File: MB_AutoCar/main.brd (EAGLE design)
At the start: 208.3 x 141 mm, 50 parts, among them K1 CQ1-12V, K2 CQ1-12V, K3 CQ1-12V, K4 CQ1-12V, Q1 PN2222, Q2 PN2222, Q3 PN2222, Q4 PN2222, U1 ARDUINO-MEGAFULL

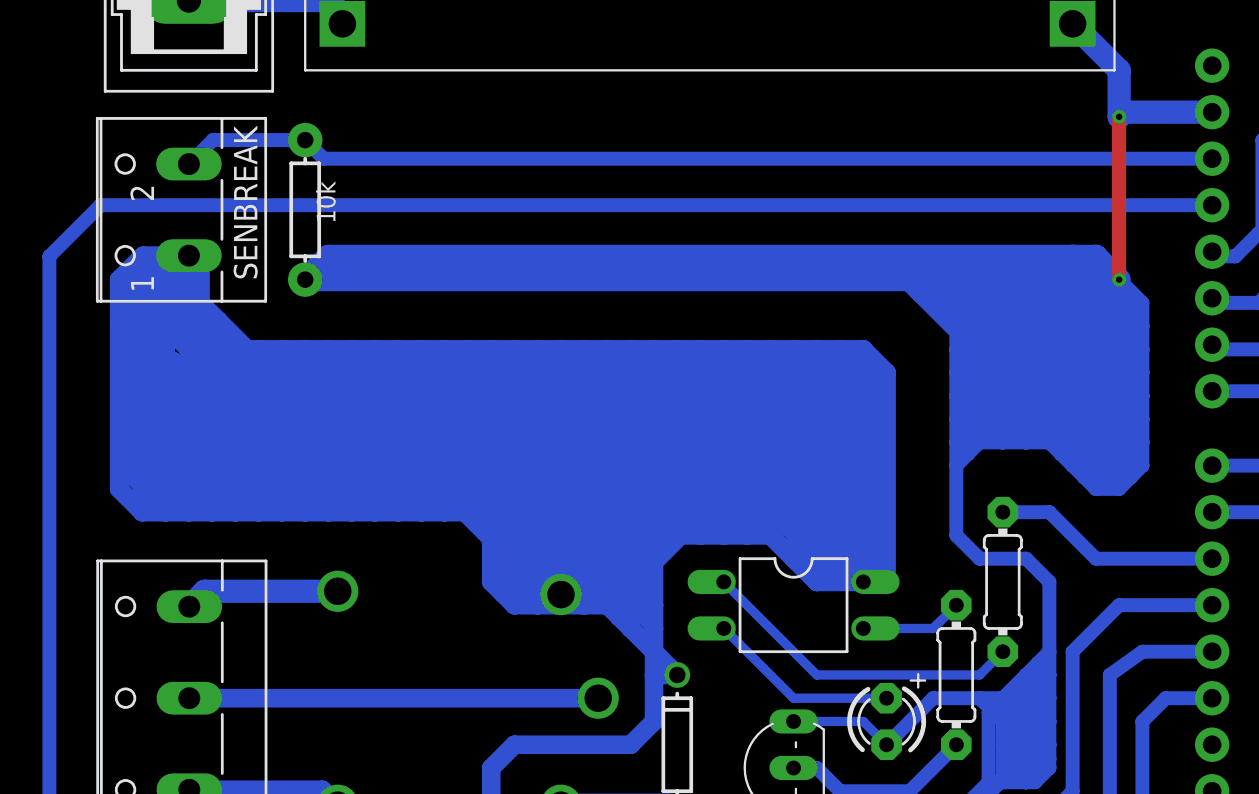
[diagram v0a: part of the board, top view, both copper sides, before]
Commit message: update
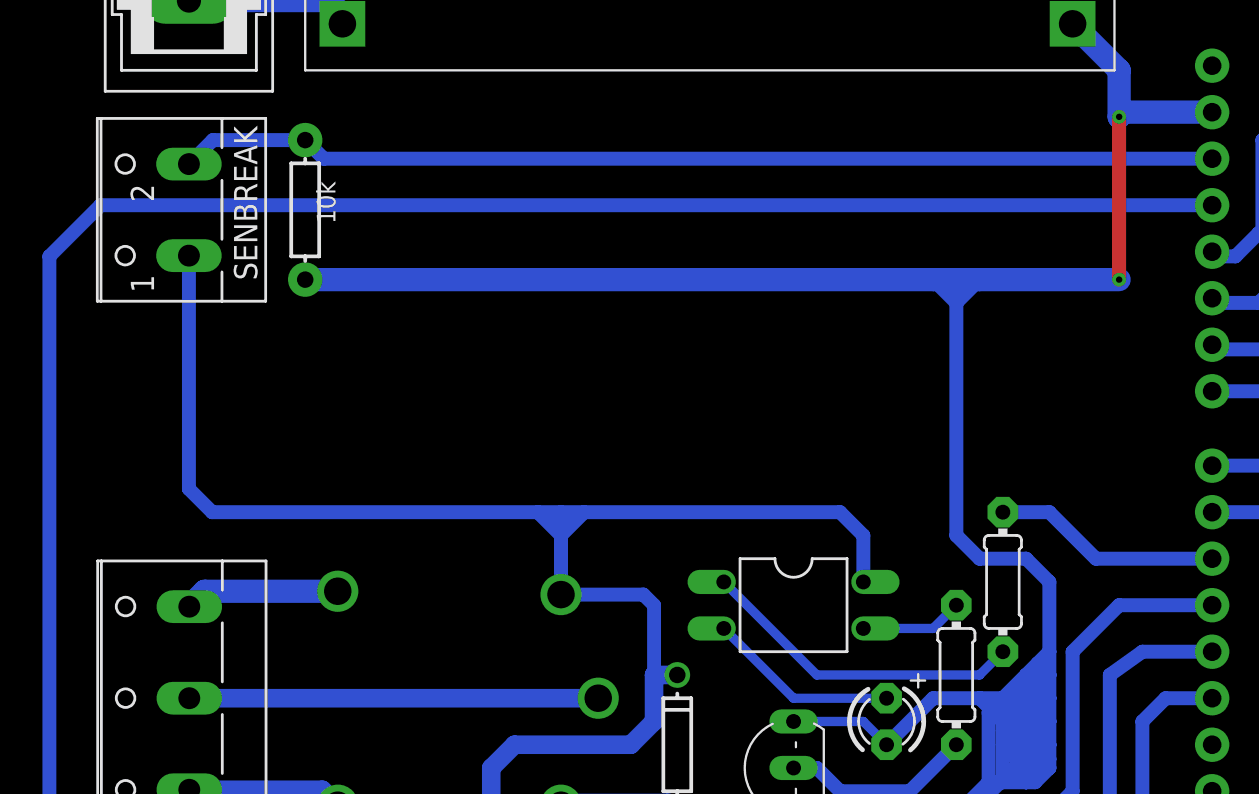
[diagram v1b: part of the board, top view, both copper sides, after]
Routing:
- net VCC: track 1448.2 -> 716.0 mm
- net GND: track 1429.5 -> 1056.0 mm
